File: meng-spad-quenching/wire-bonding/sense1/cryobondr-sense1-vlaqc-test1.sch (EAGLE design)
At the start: 30 parts, among them IC2 SENSE1, U1 SN74LVC1G34DBVT, X1 SPAD1, X10 AQCR3_VDD2V5, X11 HTR1, X12 HTR2, X2 SPAD2, X3 HTR3, X4 AQCR3_AV_DET, X5 AQCR3_IBIAS, X6 SPAD4, X7 SPAD3, X8 HTR4, X9 AQCR3_SPAD_CATHODE

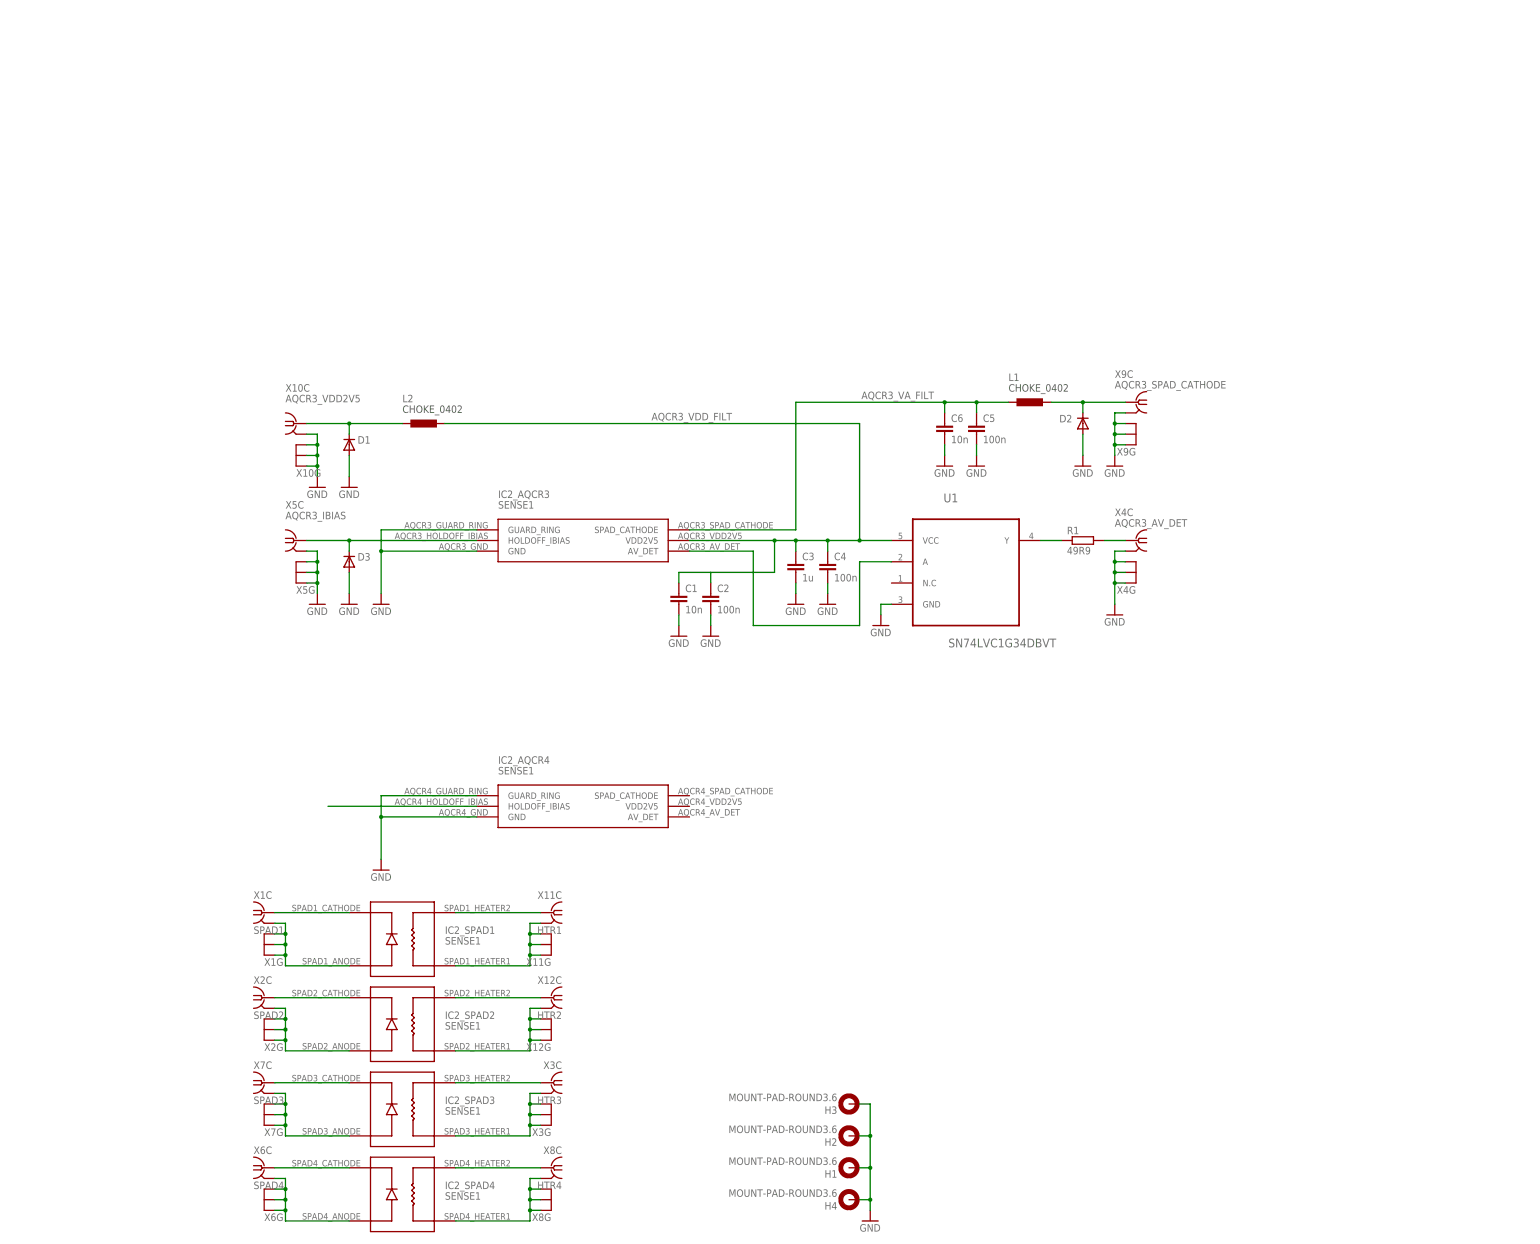
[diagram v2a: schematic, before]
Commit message: Layout done, exported first gerber
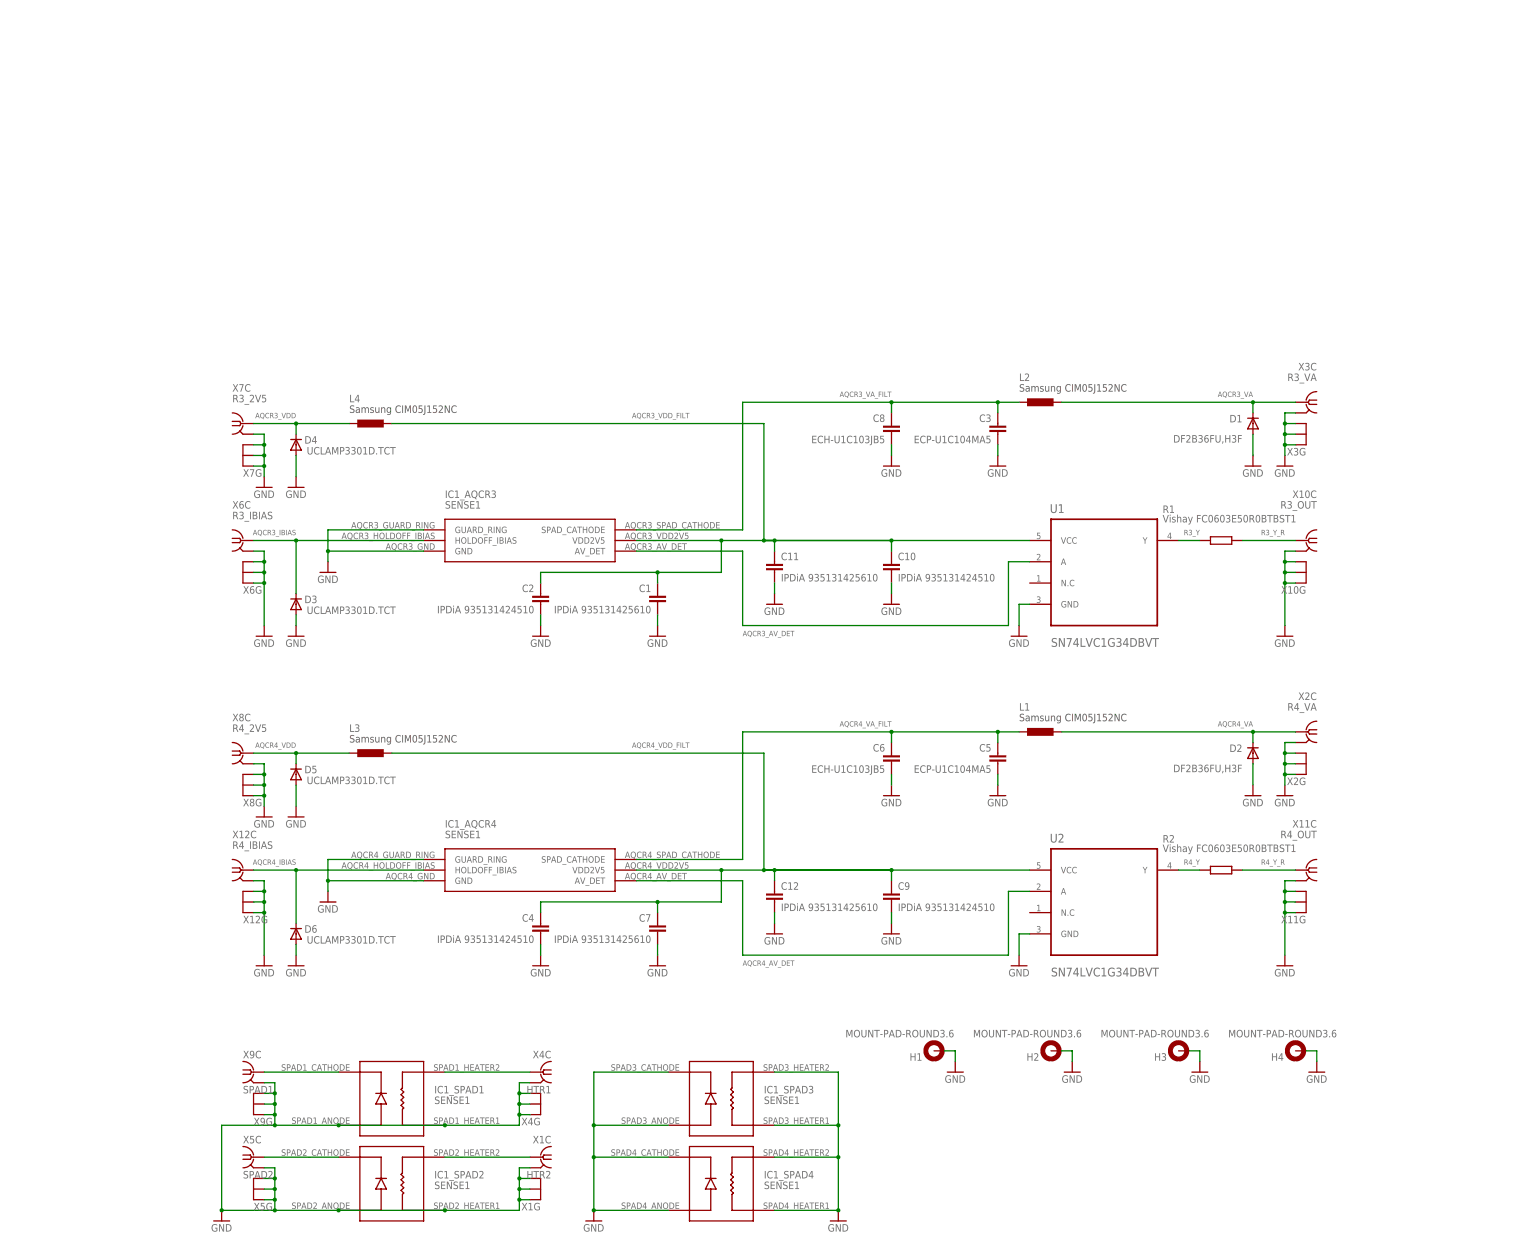
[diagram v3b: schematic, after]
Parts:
- removed IC2: SENSE1, meng:SENSE1-WIREBOND-VLAQC-TEST1
- added C10, C9: IPDiA 935131424510, rcl-modified-footprints:C-EUC0402
- added C11, C12, C7: IPDiA 935131425610, rcl-modified-footprints:C-EUC0603
- added C8: ECH-U1C103JB5, rcl-modified-footprints:C-EUC0805
- added D4, D5, D6: UCLAMP3301D.TCT, diode:DIODE-SOD323-W
- added IC1: SENSE1, meng:SENSE1-WIREBOND-VLAQC-TEST1
- added L3, L4: Samsung CIM05J152NC, meng:INDUCTOR0402
- added R2: Vishay FC0603E50R0BTBST1, rcl-modified-footprints:R-EU_R0603
- added U2: SN74LVC1G34DBVT, Texas Instruments_By_element14_Batch_1:SN74LVC1G34DBVT
- C1: value 10n -> IPDiA 935131425610
- C2, C4: value 100n -> IPDiA 935131424510; device rcl-modified-footprints:C-EUC0603 -> rcl-modified-footprints:C-EUC0402
- C3: value 1u -> ECP-U1C104MA5; device rcl-modified-footprints:C-EUC0603 -> rcl-modified-footprints:C-EUC0805
- C5: value 100n -> ECP-U1C104MA5; device rcl-modified-footprints:C-EUC0603 -> rcl-modified-footprints:C-EUC0805
- C6: value 10n -> ECH-U1C103JB5; device rcl-modified-footprints:C-EUC0603 -> rcl-modified-footprints:C-EUC0805
- D1, D2: value (none) -> DF2B36FU,H3F
- D3: value (none) -> UCLAMP3301D.TCT
- L1, L2: value CHOKE_0402 -> Samsung CIM05J152NC
- R1: value 49R9 -> Vishay FC0603E50R0BTBST1
- X1: value SPAD1 -> HTR2
- X10: value AQCR3_VDD2V5 -> R3_OUT
- X11: value HTR1 -> R4_OUT
- X12: value HTR2 -> R4_IBIAS
- X2: value SPAD2 -> R4_VA
- X3: value HTR3 -> R3_VA
- X4: value AQCR3_AV_DET -> HTR1
- X5: value AQCR3_IBIAS -> SPAD2
- X6: value SPAD4 -> R3_IBIAS
- X7: value SPAD3 -> R3_2V5
- X8: value HTR4 -> R4_2V5
- X9: value AQCR3_SPAD_CATHODE -> SPAD1
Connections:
- net N$2 renamed R3_Y
- removed net N$1: D1.C, L2.P$1, X10C.1
- removed net N$10: IC2_SPAD4.SPAD_CATHODE, X6C.1
- removed net N$11: IC2_SPAD4.SPAD_ANODE, X6C.GND, X6G.GND@1, X6G.GND@2, X6G.GND@3
- removed net N$12: IC2_SPAD3.SPAD_ANODE, X7C.GND, X7G.GND@1, X7G.GND@2, X7G.GND@3
- removed net N$13: IC2_SPAD3.SPAD_CATHODE, X7C.1
- removed net N$14: IC2_SPAD3.SPAD_HEATER2, X3C.1
- removed net N$15: IC2_SPAD4.SPAD_HEATER2, X8C.1
- removed net N$16: IC2_SPAD3.SPAD_HEATER1, X3C.GND, X3G.GND@1, X3G.GND@2, X3G.GND@3
- removed net N$17: IC2_SPAD4.SPAD_HEATER1, X8C.GND, X8G.GND@1, X8G.GND@2, X8G.GND@3
- removed net N$18: IC2_SPAD2.SPAD_CATHODE, X2C.1
- removed net N$19: IC2_SPAD2.SPAD_ANODE, X2C.GND, X2G.GND@1, X2G.GND@2, X2G.GND@3
- removed net N$20: IC2_SPAD1.SPAD_ANODE, X1C.GND, X1G.GND@1, X1G.GND@2, X1G.GND@3
- removed net N$21: IC2_SPAD1.SPAD_CATHODE, X1C.1
- removed net N$22: IC2_SPAD1.SPAD_HEATER2, X11C.1
- removed net N$23: IC2_SPAD2.SPAD_HEATER2, X12C.1
- removed net N$24: IC2_SPAD1.SPAD_HEATER1, X11C.GND, X11G.GND@1, X11G.GND@2, X11G.GND@3
- removed net N$25: IC2_SPAD2.SPAD_HEATER1, X12C.GND, X12G.GND@1, X12G.GND@2, X12G.GND@3
- removed net N$3: R1.2, X4C.1
- removed net N$4: D3.C, IC2_AQCR3.HOLDOFF_IBIAS, X5C.1
- removed net N$5: IC2_AQCR4.HOLDOFF_IBIAS
- removed net N$6: D2.C, L1.P$2, X9C.1
- removed net N$7: IC2_AQCR3.AV_DET, U1.A
- new net AQCR3_AV_DET: IC1_AQCR3.AV_DET, U1.A
- new net AQCR3_IBIAS: D3.C, IC1_AQCR3.HOLDOFF_IBIAS, X6C.1
- new net AQCR3_VA: D1.C, L2.P$2, X3C.1
- new net AQCR3_VDD: D4.C, L4.P$1, X7C.1
- new net AQCR4_AV_DET: IC1_AQCR4.AV_DET, U2.A
- new net AQCR4_IBIAS: D6.C, IC1_AQCR4.HOLDOFF_IBIAS, X12C.1
- new net AQCR4_VA: D2.C, L1.P$2, X2C.1
- new net AQCR4_VA_FILT: C5.1, C6.1, IC1_AQCR4.SPAD_CATHODE, L1.P$1
- new net AQCR4_VDD: D5.C, L3.P$1, X8C.1
- new net AQCR4_VDD_FILT: C12.1, C4.1, C7.1, C9.1, IC1_AQCR4.VDD2V5, L3.P$2, U2.VCC
- new net R3_Y_R: R1.2, X10C.1
- new net R4_Y: R2.1, U2.Y
- new net R4_Y_R: R2.2, X11C.1
- new net SPAD1_CATH: IC1_SPAD1.SPAD_CATHODE, X9C.1
- new net SPAD1_HTR: IC1_SPAD1.SPAD_HEATER2, X4C.1
- new net SPAD2_CATH: IC1_SPAD2.SPAD_CATHODE, X5C.1
- new net SPAD2_HTR: IC1_SPAD2.SPAD_HEATER2, X1C.1
- net AQCR3_VA_FILT: now also C3.1, C8.1, IC1_AQCR3.SPAD_CATHODE, L2.P$1; no longer C5.1, C6.1, IC2_AQCR3.SPAD_CATHODE, L1.P$1
- net AQCR3_VDD_FILT: now also C10.1, C11.1, IC1_AQCR3.VDD2V5, L4.P$2; no longer C3.1, C4.1, IC2_AQCR3.VDD2V5, L2.P$2
- net GND: now also C10.2, C11.2, C12.2, C7.2, C8.2, C9.2, D4.A, D5.A, D6.A, IC1_AQCR3.GND, IC1_AQCR3.GUARD_RING, IC1_AQCR4.GND, IC1_AQCR4.GUARD_RING, IC1_SPAD1.SPAD_ANODE, IC1_SPAD1.SPAD_HEATER1, IC1_SPAD2.SPAD_ANODE, IC1_SPAD2.SPAD_HEATER1, IC1_SPAD3.SPAD_ANODE, IC1_SPAD3.SPAD_CATHODE, IC1_SPAD3.SPAD_HEATER1, IC1_SPAD3.SPAD_HEATER2, IC1_SPAD4.SPAD_ANODE, IC1_SPAD4.SPAD_CATHODE, IC1_SPAD4.SPAD_HEATER1, IC1_SPAD4.SPAD_HEATER2, U2.GND, X11C.GND, X11G.GND@1, X11G.GND@2, X11G.GND@3, X12C.GND, X12G.GND@1, X12G.GND@2, X12G.GND@3, X1C.GND, X1G.GND@1, X1G.GND@2, X1G.GND@3, X2C.GND, X2G.GND@1, X2G.GND@2, X2G.GND@3, X3C.GND, X3G.GND@1, X3G.GND@2, X3G.GND@3, X6C.GND, X6G.GND@1, X6G.GND@2, X6G.GND@3, X7C.GND, X7G.GND@1, X7G.GND@2, X7G.GND@3, X8C.GND, X8G.GND@1, X8G.GND@2, X8G.GND@3; no longer IC2_AQCR3.GND, IC2_AQCR3.GUARD_RING, IC2_AQCR4.GND, IC2_AQCR4.GUARD_RING
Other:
- note added: "CAP FILM 0.01UF 16V 0805"
- note added: "CAP FILM 0.1UF 16V 0603"
- note added: "CAP SILICON 0.01UF 11V 0402"
- note added: "CAP SILICON 0.1UF 11V 0603"
- note added: "FERRITE BEAD 0402"
- note added: "Low-Temperature Component Guidelines: - Use NP0 tempco. ceramic capacitors, film capacitors, or silicon capacitors (eg. IPDiA) - Use thin-film chip resistors (eg. Vishay VSMP series)"
- note added: "RES THIN FILM 50 OHM 0603"
- note removed: "Low-Temperature Component Guidelines: - Use NP0 tempco. ceramic capacitors or silicon capacitors (eg. IPDiA) - Use thin-film chip resistors (eg. Vishay VSMP series)"
- moved on the sheet: C1, C2, C3, C4, C5, C6, D1, D2, D3, H1, H2, H3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
